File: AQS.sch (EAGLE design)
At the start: 40 parts, among them IC1 BME680, IC2 CH340G, IC4 ESPWROOM32, J1 ESP-PROG-2X3-1.27-SHROUDED, J2 M02X5-1.27-S, J3 USB-C-16P-16P, Q1 MMDT3904, Q2 2N7002

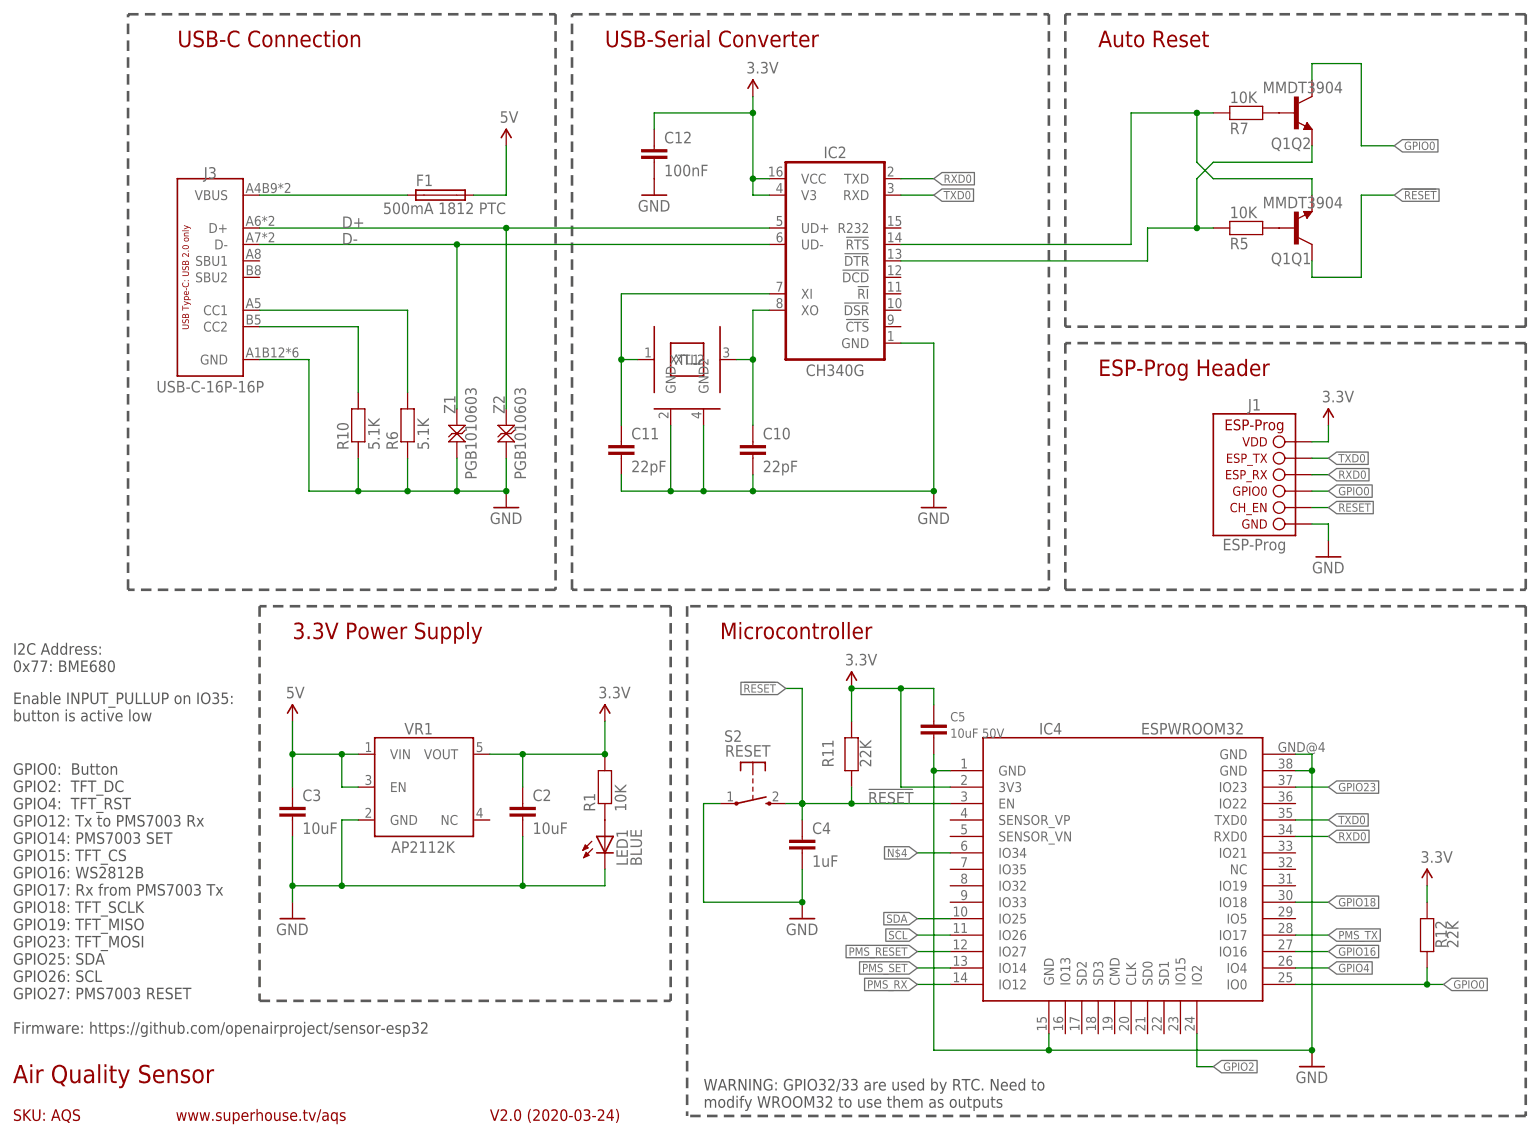
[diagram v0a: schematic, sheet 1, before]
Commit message: Replaced programming header
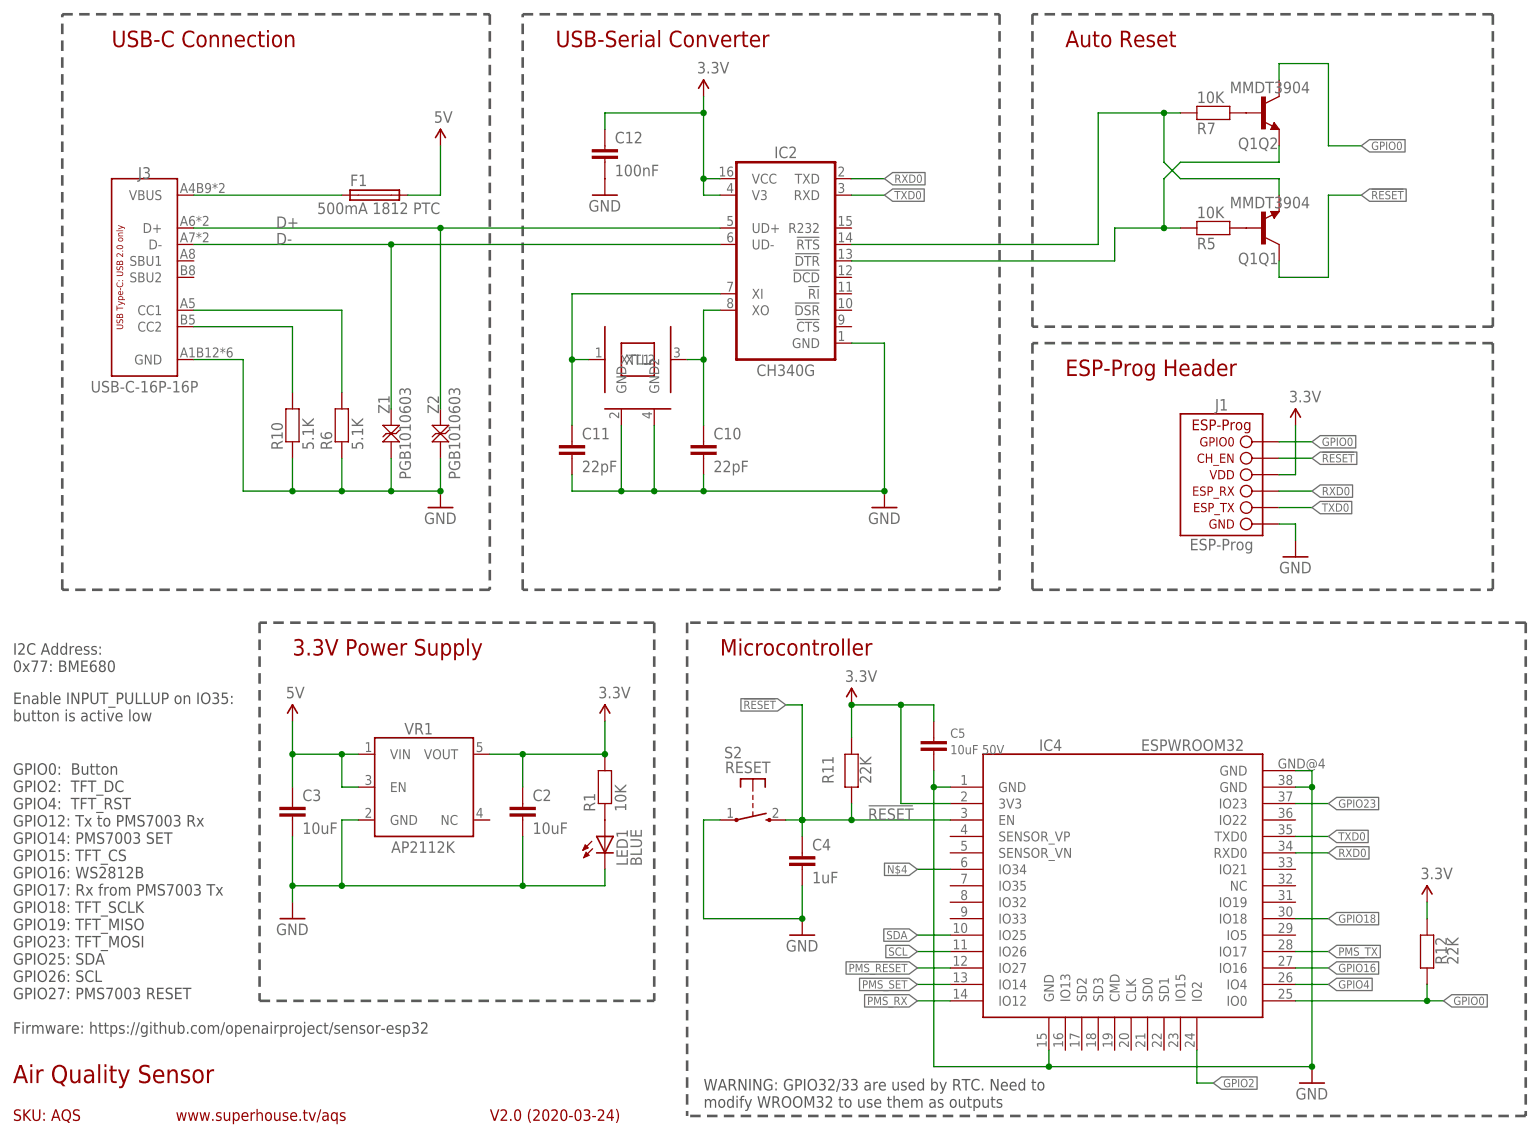
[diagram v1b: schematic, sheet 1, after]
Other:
- moved on the sheet: C10, C11, C12, C4, C5, F1, IC2, IC4, J1, J3, Q1Q1, Q1Q2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
